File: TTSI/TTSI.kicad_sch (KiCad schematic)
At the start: 35 parts, among them J101 Conn_01x02_Pin, Q101 NMOS, Q102 NMOS, Q103 NMOS, Q104 PMOS, Q106 NMOS, U1 641964-1, U101 74AHC1G32, U102 LM555xM, U103 74AHC1G08, U2 641964-1, U3 641964-1, U4 R-78E5.0-0.5, U5 641964-1

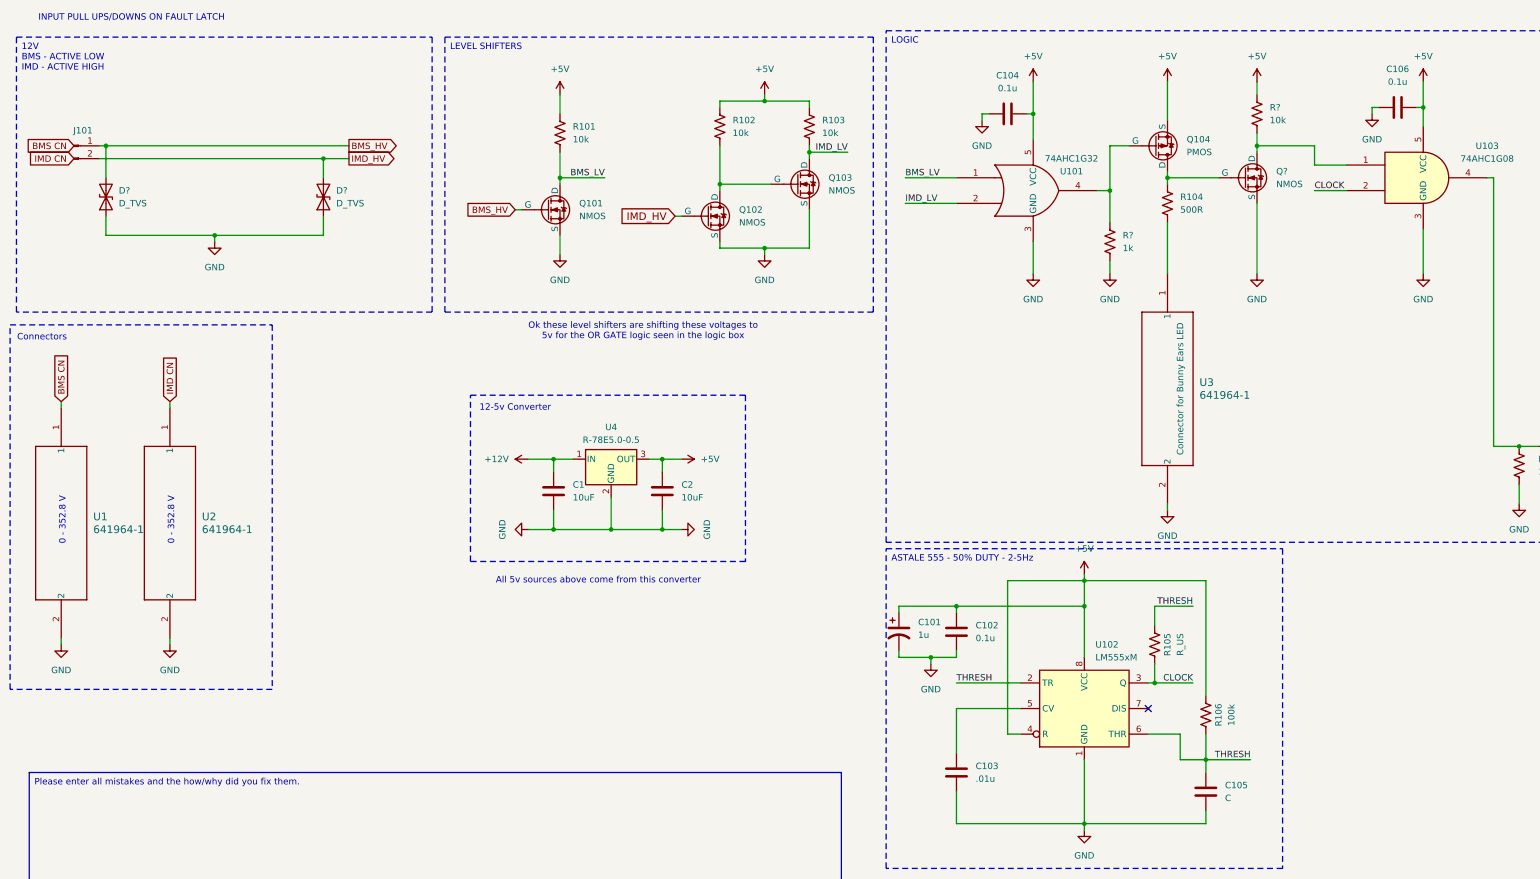
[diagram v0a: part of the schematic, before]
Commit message: RML Notes
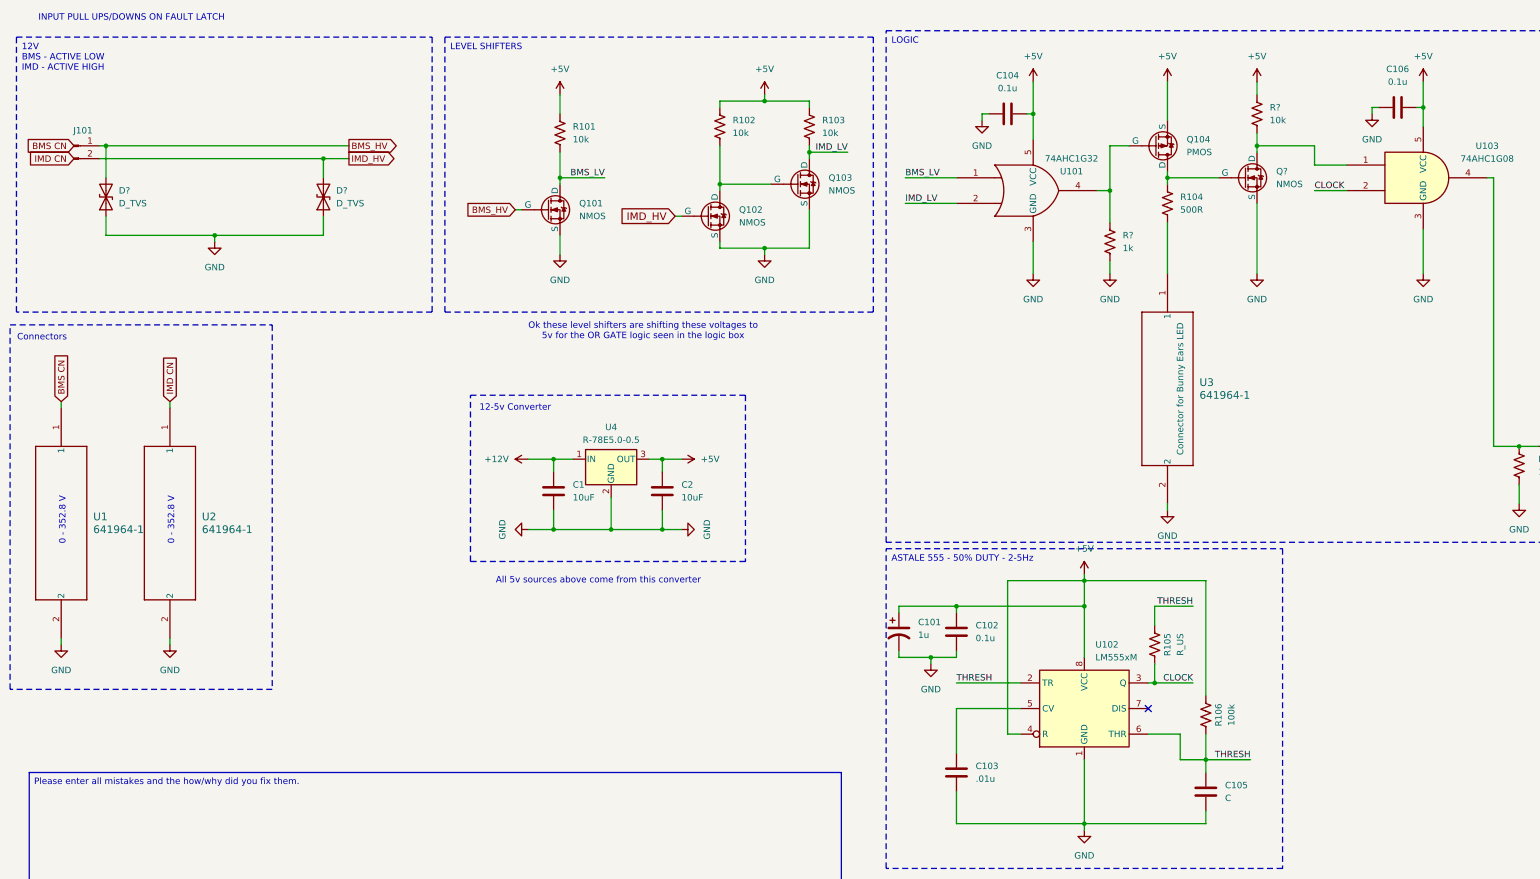
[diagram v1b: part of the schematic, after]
